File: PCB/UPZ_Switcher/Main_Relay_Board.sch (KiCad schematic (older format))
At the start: 0 parts

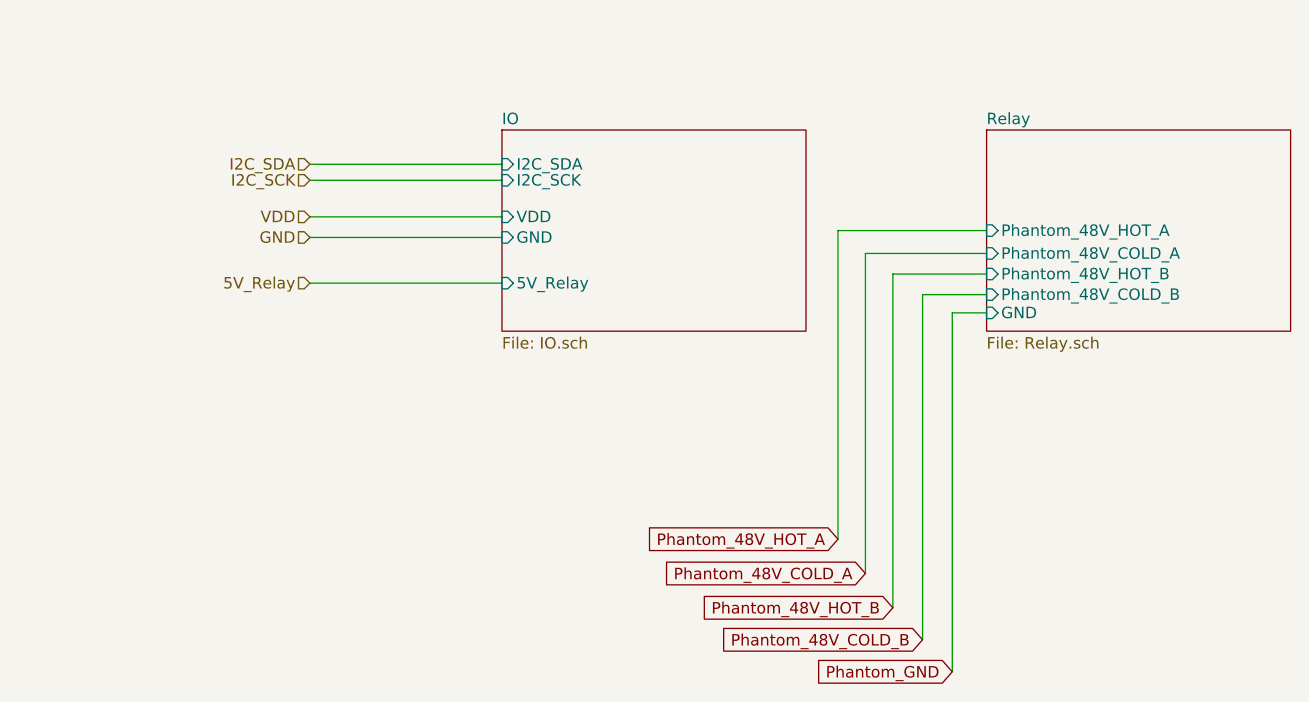
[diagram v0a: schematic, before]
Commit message: Relay Board finished
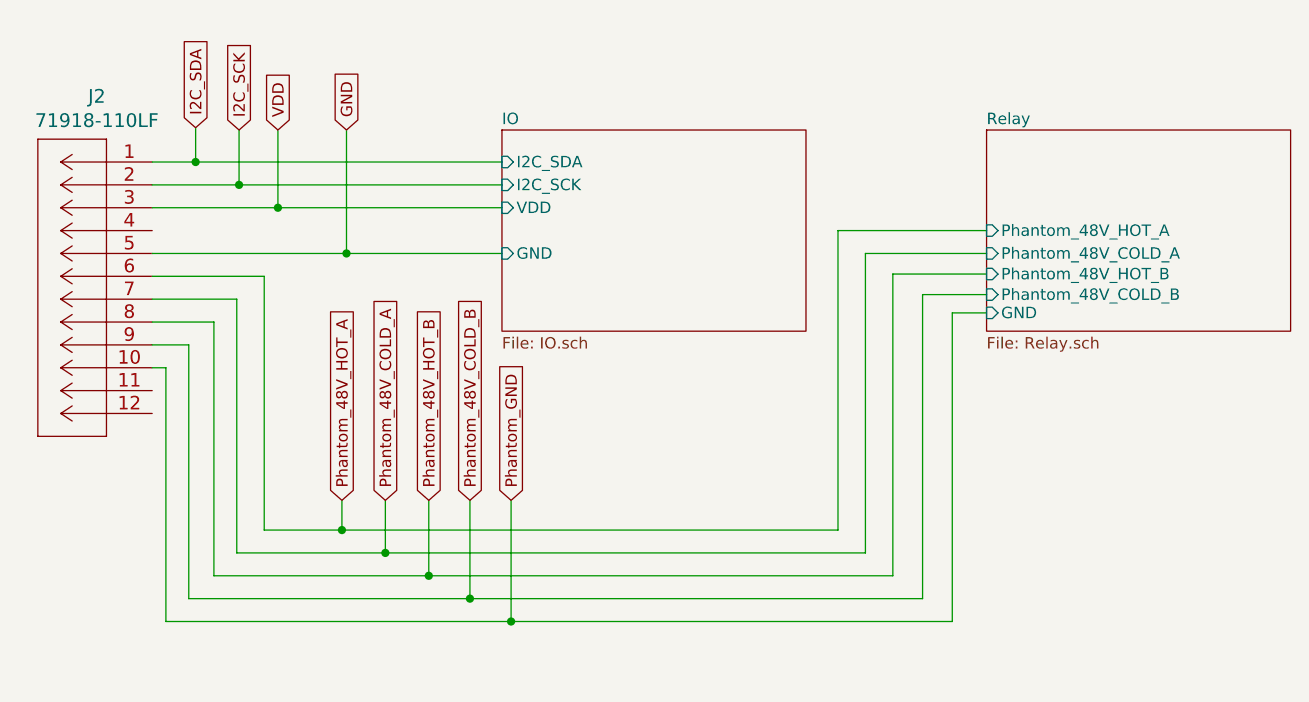
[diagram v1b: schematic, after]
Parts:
- added J2: 71918-110LF, BVKSound:71918-110LF, symbol BVKSound:71918-110LF
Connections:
- net GND: now also J2.5
- net I2C_SCK: now also J2.2
- net I2C_SDA: now also J2.1
- net Phantom_48V_COLD_A: now also J2.7
- net Phantom_48V_COLD_B: now also J2.9
- net Phantom_48V_HOT_A: now also J2.6
- net Phantom_48V_HOT_B: now also J2.8
- net Phantom_GND: now also J2.10
- net VDD: now also J2.3
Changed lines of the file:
@@
 $Descr A3 16535 11693
 encoding utf-8
-Sheet 1 3
+Sheet 1 6
 Title "IO Board"
 Date "2021-02-28"
@@
 $EndDescr
 Wire Wire Line
-	5170 4110 6010 4110
-Wire Wire Line
-	5170 4180 6010 4180
-Wire Wire Line
 	7480 4400 8130 4400
 Wire Wire Line
@@
 Wire Wire Line
 	8130 4760 7980 4760
-Wire Wire Line
-	7980 4760 7980 6330
-Text HLabel 5170 4110 0    50   Input ~ 0
-I2C_SDA
-Text HLabel 5170 4180 0    50   Input ~ 0
-I2C_SCK
-Wire Wire Line
-	5170 4340 6010 4340
-Wire Wire Line
-	5170 4430 6010 4430
-Wire Wire Line
-	5170 4630 6010 4630
-Text HLabel 5170 4340 0    50   Input ~ 0
-VDD
-Text HLabel 5170 4430 0    50   Input ~ 0
-GND
-Text HLabel 5170 4630 0    50   Input ~ 0
-5V_Relay
 $Sheet
 S 6010 3960 1330 880
@@
 F0 "IO" 50
 F1 "IO.sch" 50
-F2 "5V_Relay" I L 6010 4630 50
-F3 "I2C_SDA" I L 6010 4110 50
-F4 "I2C_SCK" I L 6010 4180 50
-F5 "VDD" I L 6010 4340 50
-F6 "GND" I L 6010 4430 50
+F2 "I2C_SDA" I L 6010 4100 50
+F3 "I2C_SCK" I L 6010 4200 50
+F4 "VDD" I L 6010 4300 50
+F5 "GND" I L 6010 4500 50
 $EndSheet
 $Sheet
@@
 F6 "Phantom_48V_COLD_B" I L 8130 4680 50
 $EndSheet
-Text GLabel 7600 5900 0    50   Input ~ 0
+Text GLabel 5500 5580 1    50   Input ~ 0
 Phantom_48V_COLD_A
-Text GLabel 7720 6050 0    50   Input ~ 0
+Text GLabel 5690 5580 1    50   Input ~ 0
 Phantom_48V_HOT_B
-Text GLabel 7850 6190 0    50   Input ~ 0
+Text GLabel 5870 5580 1    50   Input ~ 0
 Phantom_48V_COLD_B
-Text GLabel 7980 6330 0    50   Input ~ 0
+Text GLabel 6050 5580 1    50   Input ~ 0
 Phantom_GND
 Wire Wire Line
-	7600 4500 7600 5900
-Text GLabel 7480 5750 0    50   Input ~ 0
+	7600 4500 7600 5810
+Text GLabel 5310 5580 1    50   Input ~ 0
 Phantom_48V_HOT_A
 Wire Wire Line
-	7480 4400 7480 5750
+	7480 4400 7480 5710
+$Comp
+L BVKSound:71918-110LF J2
+U 1 1 604CDE14
+P 4480 4100
+F 0 "J2" H 4722 4387 60  0000 C CNN
+F 1 "71918-110LF" H 4722 4281 60  0000 C CNN
+F 2 "BVKSound:71918-110LF" H 4880 3440 60  0001 C CNN
+F 3 "" H 4480 4100 60  0000 C CNN
+	1    4480 4100
+	-1   0    0    -1
+$EndComp
+Text GLabel 4670 3950 1    50   Input ~ 0
+I2C_SDA
+Text GLabel 4860 3960 1    50   Input ~ 0
+I2C_SCK
+Text GLabel 5030 3960 1    50   Input ~ 0
+VDD
+Text GLabel 5330 3960 1    50   Input ~ 0
+GND
 Wire Wire Line
-	7720 6050 7720 4590
+	4480 4100 4670 4100
 Wire Wire Line
-	7850 6190 7850 4680
+	4670 3950 4670 4100
+Connection ~ 4670 4100
+Wire Wire Line
+	4480 4200 4860 4200
+Wire Wire Line
+	4860 3960 4860 4200
+Connection ~ 4860 4200
+Wire Wire Line
+	4480 4300 5030 4300
+Wire Wire Line
+	5030 3960 5030 4300
+Connection ~ 5030 4300
+Wire Wire Line
+	4480 4500 5330 4500
+Wire Wire Line
+	5330 3960 5330 4500
+Connection ~ 5330 4500
+Wire Wire Line
+	4970 5710 5310 5710
+Wire Wire Line
+	5310 5580 5310 5710
+Connection ~ 5310 5710
+Wire Wire Line
+	5310 5710 7480 5710
+Wire Wire Line
+	7720 5910 7720 4590
+Wire Wire Line
+	7850 6010 7850 4680
+Wire Wire Line
+	5500 5580 5500 5810
+Connection ~ 5500 5810
+Wire Wire Line
+	5500 5810 7600 5810
+Wire Wire Line
+	5690 5580 5690 5910
+Connection ~ 5690 5910
+Wire Wire Line
+	5690 5910 7720 5910
+Wire Wire Line
+	5870 5580 5870 6010
+Connection ~ 5870 6010
+Wire Wire Line
+	5870 6010 7850 6010
+Wire Wire Line
+	6050 5580 6050 6110
+Connection ~ 6050 6110
+Wire Wire Line
+	6050 6110 7980 6110
+Wire Wire Line
+	7980 4760 7980 6110
+Wire Wire Line
+	4970 4600 4970 5710
+Wire Wire Line
+	4480 4600 4970 4600
+Wire Wire Line
+	4480 4700 4850 4700
+Wire Wire Line
+	4850 4700 4850 5810
+Wire Wire Line
+	4850 5810 5500 5810
+Wire Wire Line
+	4480 4800 4750 4800
+Wire Wire Line
+	4750 4800 4750 5910
+Wire Wire Line
+	4750 5910 5690 5910
+Wire Wire Line
+	4480 4900 4640 4900
+Wire Wire Line
+	4640 4900 4640 6010
+Wire Wire Line
+	4640 6010 5870 6010
+Wire Wire Line
+	4480 5000 4540 5000
+Wire Wire Line
+	4540 5000 4540 6110
+Wire Wire Line
+	4540 6110 6050 6110
+Wire Wire Line
+	4860 4200 6010 4200
+Wire Wire Line
+	4670 4100 6010 4100
+Wire Wire Line
+	5030 4300 6010 4300
+Wire Wire Line
+	5330 4500 6010 4500
 $EndSCHEMATC

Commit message: updated phantom design + MCU board
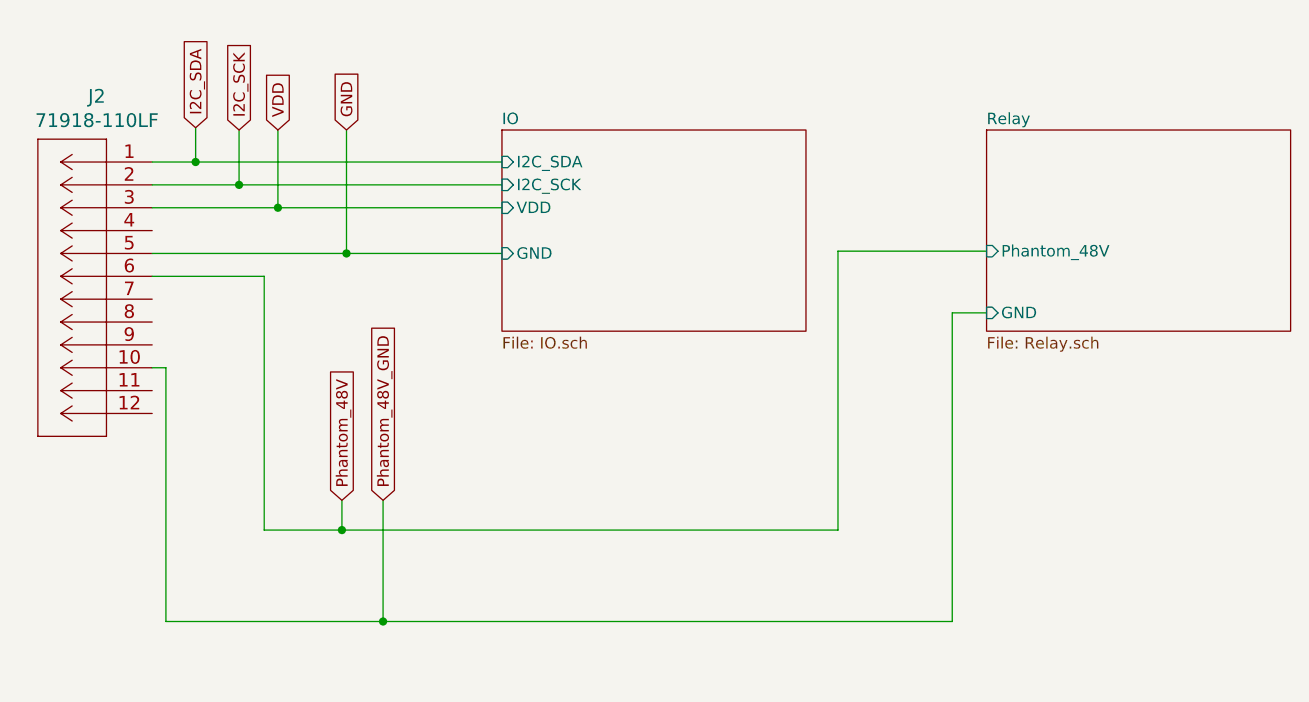
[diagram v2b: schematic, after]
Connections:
- net Phantom_48V_COLD_A: no longer names the net of J2.7
- net Phantom_48V_COLD_B: no longer names the net of J2.9
- net Phantom_48V_HOT_A renamed Phantom_48V
- net Phantom_48V_HOT_B: no longer names the net of J2.8
- net Phantom_GND renamed Phantom_48V_GND
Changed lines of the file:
@@
 $Descr A3 16535 11693
 encoding utf-8
-Sheet 1 6
+Sheet 1 3
 Title "IO Board"
 Date "2021-02-28"
@@
 Comment4 ""
 $EndDescr
-Wire Wire Line
-	7480 4400 8130 4400
-Wire Wire Line
-	8130 4500 7600 4500
-Wire Wire Line
-	7720 4590 8130 4590
-Wire Wire Line
-	7850 4680 8130 4680
 Wire Wire Line
 	8130 4760 7980 4760
@@
 F1 "Relay.sch" 50
 F2 "GND" I L 8130 4760 50
-F3 "Phantom_48V_HOT_A" I L 8130 4400 50
-F4 "Phantom_48V_COLD_A" I L 8130 4500 50
-F5 "Phantom_48V_HOT_B" I L 8130 4590 50
-F6 "Phantom_48V_COLD_B" I L 8130 4680 50
+F3 "Phantom_48V" I L 8130 4490 50
 $EndSheet
-Text GLabel 5500 5580 1    50   Input ~ 0
-Phantom_48V_COLD_A
-Text GLabel 5690 5580 1    50   Input ~ 0
-Phantom_48V_HOT_B
-Text GLabel 5870 5580 1    50   Input ~ 0
-Phantom_48V_COLD_B
-Text GLabel 6050 5580 1    50   Input ~ 0
-Phantom_GND
-Wire Wire Line
-	7600 4500 7600 5810
+Text GLabel 5490 5580 1    50   Input ~ 0
+Phantom_48V_GND
 Text GLabel 5310 5580 1    50   Input ~ 0
-Phantom_48V_HOT_A
-Wire Wire Line
-	7480 4400 7480 5710
+Phantom_48V
 $Comp
 L BVKSound:71918-110LF J2
@@
 	5310 5710 7480 5710
 Wire Wire Line
-	7720 5910 7720 4590
-Wire Wire Line
-	7850 6010 7850 4680
-Wire Wire Line
-	5500 5580 5500 5810
-Connection ~ 5500 5810
-Wire Wire Line
-	5500 5810 7600 5810
-Wire Wire Line
-	5690 5580 5690 5910
-Connection ~ 5690 5910
-Wire Wire Line
-	5690 5910 7720 5910
-Wire Wire Line
-	5870 5580 5870 6010
-Connection ~ 5870 6010
-Wire Wire Line
-	5870 6010 7850 6010
-Wire Wire Line
-	6050 5580 6050 6110
-Connection ~ 6050 6110
-Wire Wire Line
-	6050 6110 7980 6110
+	5490 5580 5490 6110
 Wire Wire Line
 	7980 4760 7980 6110
@@
 	4480 4600 4970 4600
 Wire Wire Line
-	4480 4700 4850 4700
-Wire Wire Line
-	4850 4700 4850 5810
-Wire Wire Line
-	4850 5810 5500 5810
-Wire Wire Line
-	4480 4800 4750 4800
-Wire Wire Line
-	4750 4800 4750 5910
-Wire Wire Line
-	4750 5910 5690 5910
-Wire Wire Line
-	4480 4900 4640 4900
-Wire Wire Line
-	4640 4900 4640 6010
-Wire Wire Line
-	4640 6010 5870 6010
-Wire Wire Line
 	4480 5000 4540 5000
 Wire Wire Line
 	4540 5000 4540 6110
 Wire Wire Line
-	4540 6110 6050 6110
+	4540 6110 5490 6110
 Wire Wire Line
 	4860 4200 6010 4200
@@
 Wire Wire Line
 	5330 4500 6010 4500
+Connection ~ 5490 6110
+Wire Wire Line
+	5490 6110 7980 6110
+Wire Wire Line
+	8130 4490 7480 4490
+Wire Wire Line
+	7480 4490 7480 5710
 $EndSCHEMATC
